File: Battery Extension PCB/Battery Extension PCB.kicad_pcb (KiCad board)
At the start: 2 copper layers, 76.5 x 16.7 mm, 35 parts, among them P1 Solder_Pad, P10 Solder_Pad, P11 Solder_Pad, P12 Solder_Pad, P13 Solder_Pad, P14 Solder_Pad, P2 Solder_Pad, P3 Solder_Pad, P4 Solder_Pad, P5 Solder_Pad, P6 Solder_Pad, P7 Solder_Pad, P8 Solder_Pad, P9 Solder_Pad, U1 M1250RS-02P, U3 FS8205A, U4 TPS61032PWPR, U5 TP4056, U6 DW01A, U7 FXL0530-6R8-M, U8 AP40P05

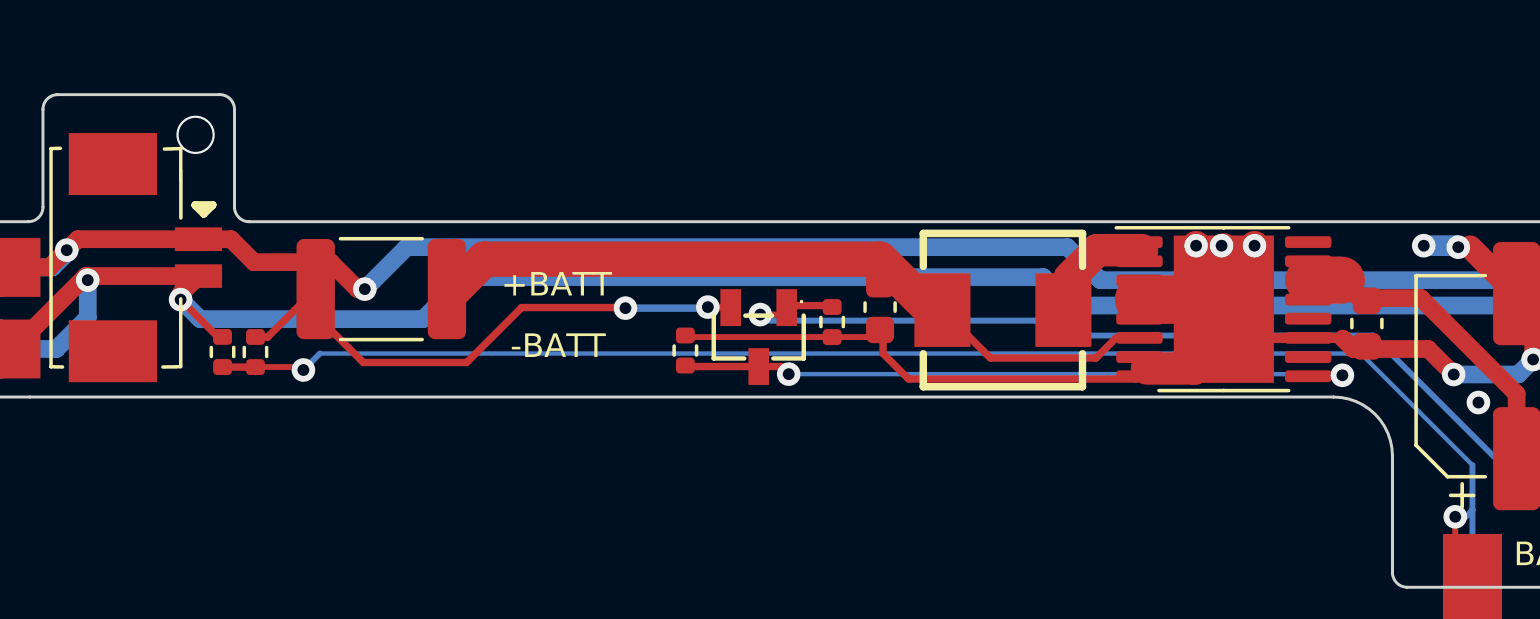
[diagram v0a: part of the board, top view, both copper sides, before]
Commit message: updated pcb designs
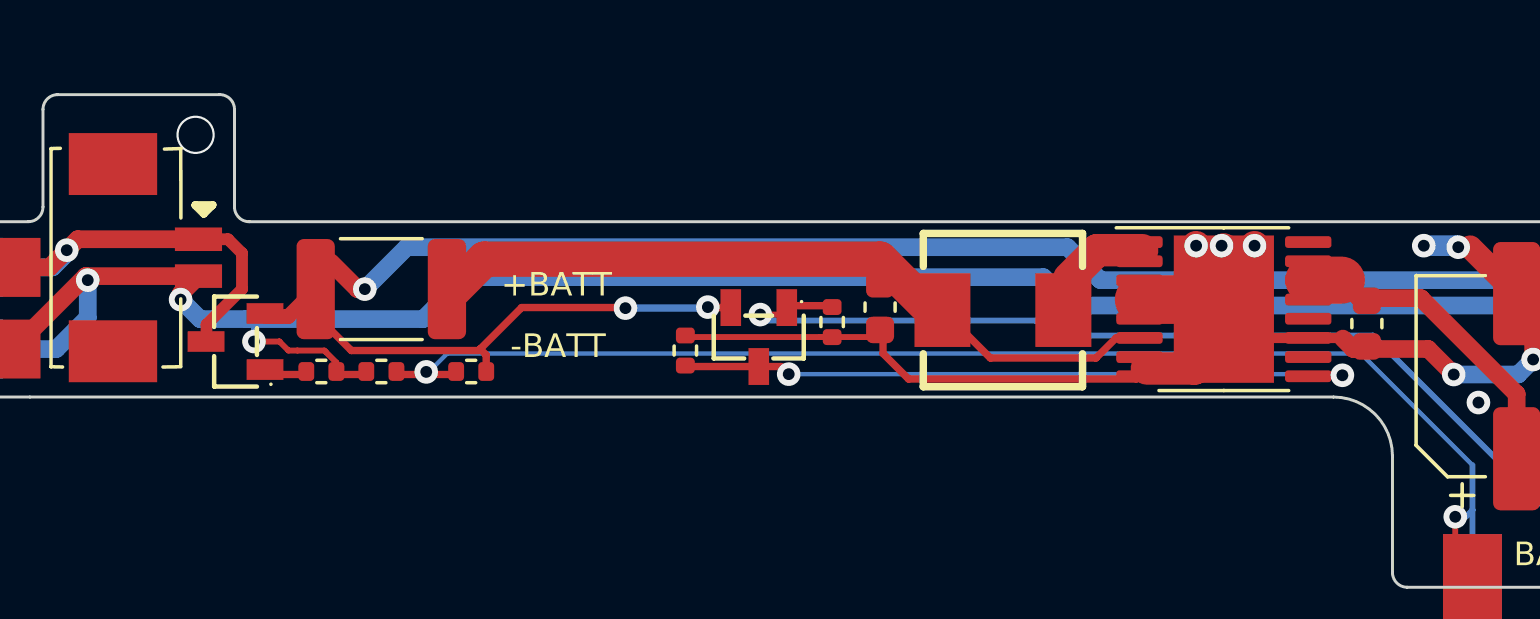
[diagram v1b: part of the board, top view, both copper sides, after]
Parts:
- added R3: 100K, Resistor_SMD:R_0402_1005Metric, F.Cu at (79.3, 73.5)
- added U2: AP40P05, footprint:SOT-23-3_L2.9-W1.3-P1.90-LS2.4-BR, F.Cu at (76.4, 72.4)
- R1: value 100K -> 33K
- moved R1 7.34 mm to (84.4, 73.5), turned to 0 degrees
- moved R2 5.43 mm to (81.3, 73.5), turned to 0 degrees
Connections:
- P1 pad 1: +BATT -> Net-(P1-Pad1)
- P8 pad 1: +BATT -> Net-(P1-Pad1)
- U1 pad 1: +BATT -> Net-(P1-Pad1)
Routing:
- net Net-(P1-Pad1): track 0.00 -> 17.2 mm, vias 0 -> 1
- net +BATT: track 91.8 -> 75.1 mm, vias 5 -> 4
- net BATT VOLT: track 51.7 -> 46.8 mm
- net -BATT: track 89.0 -> 92.3 mm, vias 7 -> 8
- net Net-(R3-Pad2): track 0.00 -> 1.41 mm
